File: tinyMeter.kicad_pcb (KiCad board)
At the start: 2 copper layers, 74.6 x 70 mm, 93 parts, among them J1 USB_MASTER, J2 DC_POWER, J3 USB_POWER, J4 USBA_OUT_2, J5 USBA_OUT_1, J6 DC_POWER, J7 Debug, J8 External antenna, Q1 100N03A, Q2 100N03A, Q3 100N03A, Q4 SS8050, SW1 SW_Push, SW2 SW_Push, SW3 SW_Push, SW4 SW_Push, SW5 SW_Push, SW6 Boot, SW7 Reset, U1 ESP32-S3, U2 INA219AxD, U3 INA219AxD, U4 INA219AxD, U5 AMS1117-3.3, Y1 Crystal_GND24

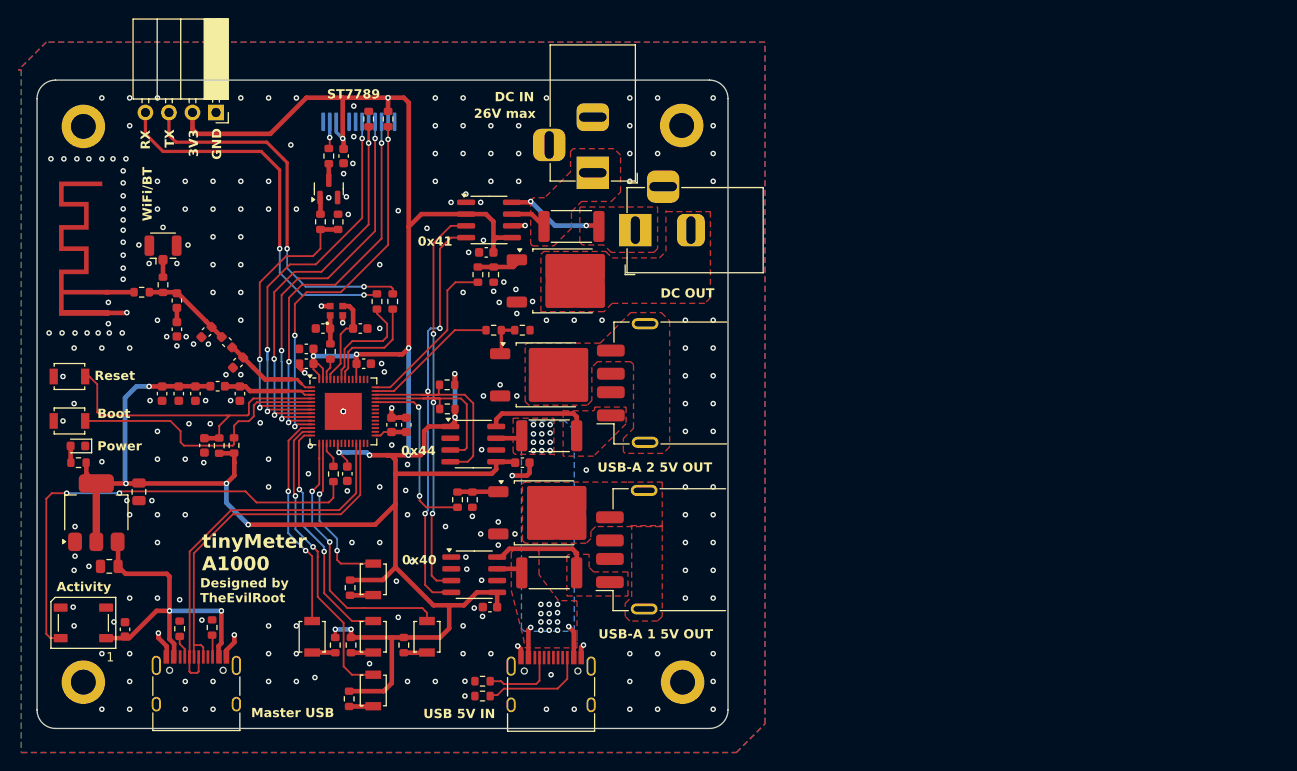
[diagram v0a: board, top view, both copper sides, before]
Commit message: Working on v2
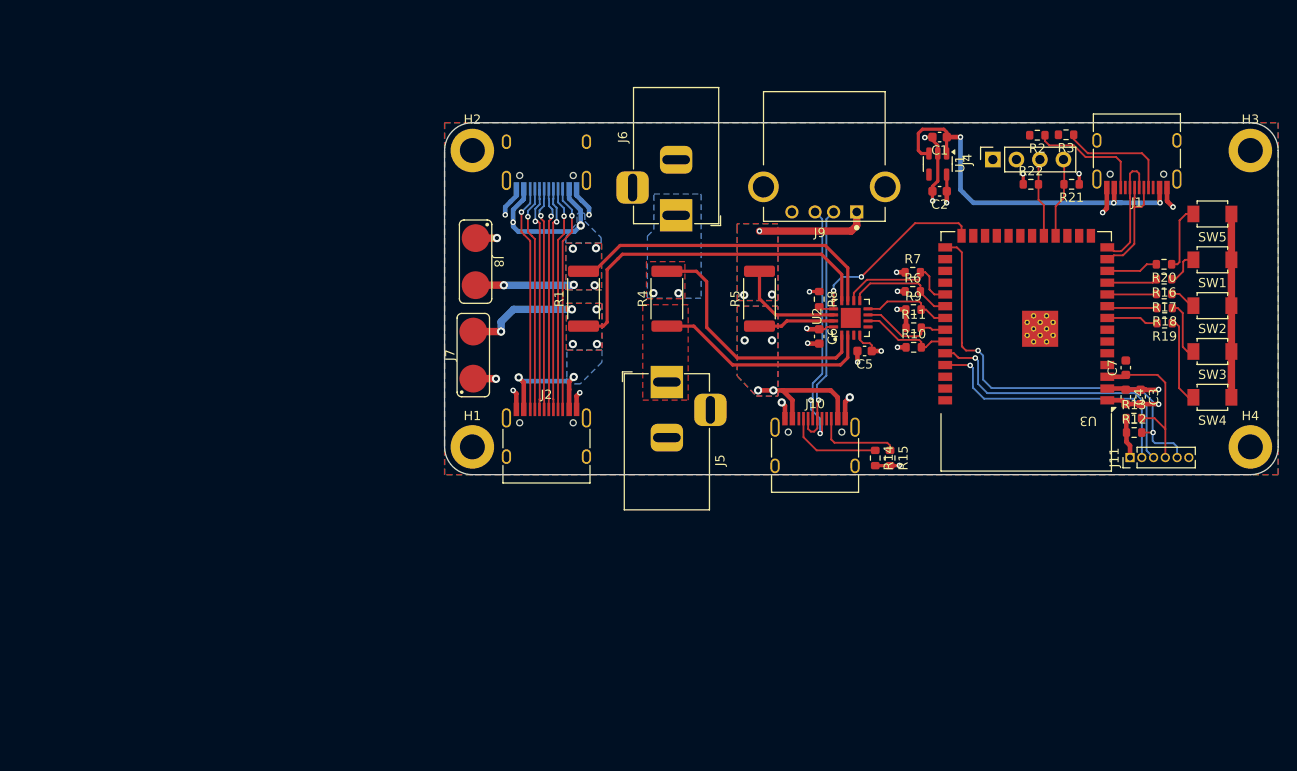
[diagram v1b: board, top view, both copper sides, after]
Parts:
- removed AE1: PCB antenna, Library:ESPRESSIF_ESP32_MIFA_2.4GHz_Right
- removed C10, C11, C16, C17, C19, C20, C21, C22, C23: 100n, Capacitor_SMD:C_0603_1608Metric
- removed C12, C15, C18: 1u, Capacitor_SMD:C_0603_1608Metric
- removed C13, C14: 10u, Capacitor_SMD:C_0603_1608Metric
- removed C8, C9: LNA, Capacitor_SMD:C_0603_1608Metric
- removed D1: WS2812B, LED_SMD:LED_WS2812B_PLCC4_5.0x5.0mm_P3.2mm
- removed D2: PWR_LED, LED_SMD:LED_0603_1608Metric
- removed DS1: ST77xx, Library:ST77XX
- removed L1, L2: L, Inductor_SMD:L_0603_1608Metric
- removed L3: 2n, Inductor_SMD:L_0603_1608Metric
- removed Q1, Q2, Q3: 100N03A, Package_TO_SOT_SMD:TO-252-2
- removed Q4: SS8050, Package_TO_SOT_SMD:SOT-23
- removed R23, R31: 1k, Resistor_SMD:R_0603_1608Metric
- removed R24, R25, R28, R32, R33, R34: 10k, Resistor_SMD:R_0603_1608Metric
- removed R26, R27: 2k7, Resistor_SMD:R_0603_1608Metric
- removed R29: 60, Resistor_SMD:R_0603_1608Metric
- removed R30: 100, Resistor_SMD:R_0603_1608Metric
- removed SW6: Boot, Button_Switch_SMD:SW_SPST_B3U-1000P
- removed SW7: Reset, Button_Switch_SMD:SW_SPST_B3U-1000P
- removed U4: INA219AxD, Package_SO:SOIC-8_3.9x4.9mm_P1.27mm
- removed U5: AMS1117-3.3, Package_TO_SOT_SMD:SOT-223-3_TabPin2
- removed Y1: Crystal_GND24, Library:OSC_XRCGB40M000F4M00R0
- added J10: USB_IN, TheEvilRoot:USB_C_Receptacle_HRO_TYPE-C-31-M-12, F.Cu at (223.0, 115.0)
- added J11: Conn_01x06, Connector_PinHeader_1.27mm:PinHeader_1x06_P1.27mm_Vertical, F.Cu at (257.0, 115.2)
- added J9: USB_OUT, TheEvilRoot:TE_292303-1, F.Cu at (227.5, 88.6)
- C1, C2: footprint Capacitor_SMD:C_0805_2012Metric -> Capacitor_SMD:C_0603_1608Metric
- C3: value 10u -> 1u
- C4, C5: value 10p -> 100n
- C6: value 10u -> 100n
- C7: value LNA -> 10u
- J1: value USB_MASTER -> USB_C_Receptacle_USB2.0_16P; footprint Connector_USB:USB_C_Receptacle_HRO_TYPE-C-31-M-12 -> TheEvilRoot:USB_C_Receptacle_HRO_TYPE-C-31-M-12
- J2: value DC_POWER -> USB_IN; footprint Connector_BarrelJack:BarrelJack_Horizontal -> TheEvilRoot:USB_C_Receptacle_HRO_TYPE-C-31-M-12
- J3: value USB_POWER -> USB_OUT; footprint Connector_USB:USB_C_Receptacle_HRO_TYPE-C-31-M-12 -> TheEvilRoot:USB_C_Receptacle_HRO_TYPE-C-31-M-12; moved to B.Cu
- J4: value USBA_OUT_2 -> OLED; footprint Connector_USB:USB_A_Receptacle_GCT_USB1046 -> Connector_PinSocket_2.54mm:PinSocket_1x04_P2.54mm_Vertical
- J5: value USBA_OUT_1 -> DC_IN; footprint Connector_USB:USB_A_Receptacle_GCT_USB1046 -> Connector_BarrelJack:BarrelJack_Horizontal
- J6: value DC_POWER -> DC_OUT
- J7: value Debug -> Conn_01x02; footprint Connector_PinSocket_2.54mm:PinSocket_1x04_P2.54mm_Horizontal -> TheEvilRoot:SolderWire-SMD-2pin-2.54mm-D3.0
- J8: value External antenna -> Conn_01x02; footprint Connector_Coaxial:U.FL_Hirose_U.FL-R-SMT-1_Vertical -> TheEvilRoot:SolderWire-SMD-2pin-2.54mm-D3.0
- R1, R4: value 5k1 -> R100; footprint Resistor_SMD:R_0603_1608Metric -> Resistor_SMD:R_2512_6332Metric
- R10, R6, R7, R9: value 0R -> 10k
- R11, R8: value R025 -> 10k; footprint Resistor_SMD:R_2512_6332Metric -> Resistor_SMD:R_0603_1608Metric
- R12, R13: value 220 -> 10k
- R14, R15: value 10k -> 5k1
- R16, R17, R18, R19: value 10k -> R
- R20: value 1k -> R
- R21: value 1k -> 2k7
- R22: value 10k -> 2k7
- R5: value R025 -> R100
- SW1: value SW_Push -> A1; footprint Button_Switch_SMD:SW_SPST_B3U-1000P -> TheEvilRoot:IT-1185AP
- SW2: value SW_Push -> A2; footprint Button_Switch_SMD:SW_SPST_B3U-1000P -> TheEvilRoot:IT-1185AP
- SW3: value SW_Push -> A3; footprint Button_Switch_SMD:SW_SPST_B3U-1000P -> TheEvilRoot:IT-1185AP
- SW4: value SW_Push -> A4; footprint Button_Switch_SMD:SW_SPST_B3U-1000P -> TheEvilRoot:IT-1185AP
- SW5: value SW_Push -> A0; footprint Button_Switch_SMD:SW_SPST_B3U-1000P -> TheEvilRoot:IT-1185AP
- U1: value ESP32-S3 -> AP2112K-3.3; footprint Package_DFN_QFN:QFN-56-1EP_7x7mm_P0.4mm_EP4x4mm -> Package_TO_SOT_SMD:SOT-23-5
- U2: value INA219AxD -> INA3221AIRGVR; footprint Package_SO:SOIC-8_3.9x4.9mm_P1.27mm -> TheEvilRoot:QFN65P400X400X100-17N
- U3: value INA219AxD -> ESP32-S3-WROOM-1; footprint Package_SO:SOIC-8_3.9x4.9mm_P1.27mm -> TheEvilRoot:ESP32-S3-WROOM-1
- moved H3 138.5 mm to (270.0, 82.0)
- moved J1 117.3 mm to (257.8, 82.0), turned to 180 degrees
- moved R13 114.1 mm to (257.4, 110.9), turned to 0 degrees
- moved R2 106.8 mm to (247.0, 80.3), turned to 180 degrees
- moved SW5 104.2 mm to (265.9, 88.8), turned to 180 degrees
- moved C3 101.2 mm to (258.1, 108.6)
- moved C1 100.9 mm to (236.4, 80.5)
- moved SW4 100.6 mm to (265.9, 108.7), turned to 180 degrees
- moved R18 97.6 mm to (260.8, 99.0), turned to 180 degrees
- moved R17 97.2 mm to (260.7, 97.5), turned to 180 degrees
- moved SW1 96.9 mm to (265.9, 93.8), turned to 180 degrees
- moved R16 96.3 mm to (260.7, 95.9), turned to 180 degrees
- moved C7 95.9 mm to (256.6, 105.5), turned to 90 degrees
- moved SW3 95.7 mm to (265.9, 103.7), turned to 180 degrees
- moved C2 92.3 mm to (236.4, 86.4), turned to 180 degrees
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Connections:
- C1 pad 1: USB_VBUS -> VBUS
- C3 pad 1: /ESP_EN -> +3V3
- C4 pad 1: /ESP_XTAL_N -> +3V3
- C5 pad 1: /ESP_XTAL_IN -> +3V3
- C7 pad 1: /ESP_LNA -> /ESP_EN
- J1 pad A4: USB_VBUS -> VBUS
- J1 pad A9: USB_VBUS -> VBUS
- J1 pad B4: USB_VBUS -> VBUS
- J1 pad B9: USB_VBUS -> VBUS
- J3 pad A4: PWR_5V -> /METER_1-
- J3 pad A5: /USB_POWER_CC1 -> /USB_C_CC1
- J3 pad A6: unconnected-(J3-D+-PadA6) -> /USB_C_D2+
- J3 pad A7: unconnected-(J3-D--PadA7) -> /USB_C_D1-
- J3 pad A8: unconnected-(J3-SBU1-PadA8) -> /USB_C_SBU1
- J3 pad A9: PWR_5V -> /METER_1-
- J3 pad B4: PWR_5V -> /METER_1-
- J3 pad B5: /USB_POWER_CC2 -> /USB_C_CC2
- J3 pad B6: unconnected-(J3-D+-PadB6) -> /USB_C_D1+
- J3 pad B7: unconnected-(J3-D--PadB7) -> /USB_C_D2-
- J3 pad B8: unconnected-(J3-SBU2-PadB8) -> /USB_C_SBU2
- J3 pad B9: PWR_5V -> /METER_1-
- J4 pad 1: /USBA_OUT2_VCC -> GND
- J4 pad 2: unconnected-(J4-D--Pad2) -> +3V3
- J4 pad 3: unconnected-(J4-D+-Pad3) -> /OLED_SCL
- J4 pad 4: /USBA_OUT2_GND -> /OLED_SDA
- J5 pad 1: /USBA_OUT1_VCC -> /METER_3+
- J5 pad 2: unconnected-(J5-D--Pad2) -> GND
- J5 pad 3: unconnected-(J5-D+-Pad3) -> (no net)
- J6 pad 1: /DC_POWER_VCC -> /METER_3-
- J6 pad 2: /DC_POWER_GND -> GND
- J7 pad 2: +3V3 -> /METER_1+
- J8 pad 1: /WIFI_ANTENNA_EXT -> GND
- J8 pad 2: GND -> /METER_1-
- R1 pad 1: GND -> /METER_1+
- R1 pad 2: /USB_MASTER_CC2 -> /METER_1-
- R10 pad 1: /WIFI_ANTENNA -> +3V3
- R10 pad 2: /WIFI_ANTENNA_EXT -> /METER_SCL
- R11 pad 1: /DC_POWER_VCC -> +3V3
- R11 pad 2: PWR_DC -> /METER_SDA
- R12 pad 1: /MCU_LED_DIN -> +3V3
- R12 pad 2: /MCU_LED_DATA -> /ESP_BOOT
- R13 pad 2: /3V3_PWR_LED -> /ESP_EN
- R14 pad 1: Net-(R14-Pad1) -> /USB_A_CC1
- R14 pad 2: +3V3 -> GND
- R15 pad 1: Net-(R15-Pad1) -> /USB_A_CC2
- R15 pad 2: +3V3 -> GND
- R16 pad 2: +3V3 -> /SW_A1
- R17 pad 2: +3V3 -> /SW_A2
- R18 pad 2: +3V3 -> /SW_A3
- R19 pad 1: /USBA_OUT1_GATE -> Net-(R19-Pad1)
- R19 pad 2: GND -> /SW_A4
- R2 pad 1: GND -> /USB_MASTER_CC2
- R2 pad 2: /USB_MASTER_CC1 -> GND
- R20 pad 1: /USBA_OUT1_GATE -> Net-(R20-Pad1)
- R20 pad 2: /USBA_OUT_1_FETGATE -> /SW_A0
- R21 pad 1: /USBA_OUT2_GATE -> +3V3
- R21 pad 2: /USBA_OUT_2_FETGATE -> /OLED_SDA
- R22 pad 1: /USBA_OUT2_GATE -> +3V3
- R22 pad 2: GND -> /OLED_SCL
- R3 pad 1: GND -> /USB_MASTER_CC1
- R3 pad 2: /USB_POWER_CC2 -> GND
- R4 pad 1: GND -> /METER_3+
- R4 pad 2: /USB_POWER_CC1 -> /METER_3-
- R5 pad 1: /USBA_OUT1_VCC -> /METER_2+
- R5 pad 2: PWR_5V -> /METER_2-
- R6 pad 1: /ESP_TX -> +3V3
- R6 pad 2: /ESP_TDX0 -> /METER_CRIT
- R7 pad 1: /ESP_RX -> +3V3
- R7 pad 2: /ESP_RDX0 -> /METER_VALID
- R8 pad 1: /USBA_OUT2_VCC -> +3V3
- R8 pad 2: PWR_5V -> /METER_TIMING
- R9 pad 1: /WIFI_ANTENNA -> +3V3
- R9 pad 2: /WIFI_ANTENNA_PCB -> /METER_WARN
- SW1 pad 1: /KEYPAD_K1 -> +3V3
- SW1 pad 2: Net-(R14-Pad1) -> Net-(R16-Pad1)
- SW2 pad 1: /KEYPAD_K2 -> +3V3
- SW2 pad 2: Net-(R15-Pad1) -> Net-(R17-Pad1)
- SW3 pad 1: /KEYPAD_K3 -> +3V3
- SW3 pad 2: Net-(R16-Pad1) -> Net-(R18-Pad1)
- SW4 pad 1: /KEYPAD_K4 -> +3V3
- SW4 pad 2: Net-(R17-Pad1) -> Net-(R19-Pad1)
- SW5 pad 1: /KEYPAD_K5 -> +3V3
- SW5 pad 2: Net-(R18-Pad1) -> Net-(R20-Pad1)
- U1 pad 1: /ESP_LNA -> VBUS
- U1 pad 2: /ESP_VDD_3P3 -> GND
- U1 pad 3: /ESP_VDD_3P3 -> VBUS
- U1 pad 4: /ESP_EN -> unconnected-(U1-NC-Pad4)
- U1 pad 5: /ESP_IO0 -> +3V3
- U2 pad 1: GND -> /METER_3-
- U2 pad 2: GND -> /METER_3+
- U2 pad 3: /METER_SDA -> GND
- U2 pad 4: /METER_SCL -> +3V3
- U2 pad 5: +3V3 -> GND
- U2 pad 6: GND -> /METER_SCL
- U2 pad 7: PWR_5V -> /METER_SDA
- U2 pad 8: /USBA_OUT1_VCC -> /METER_WARN
- U3 pad 1: +3V3 -> GND
- U3 pad 2: GND -> +3V3
- U3 pad 3: /METER_SDA -> /ESP_EN
- U3 pad 4: /METER_SCL -> unconnected-(U3-IO4-Pad4)
- U3 pad 5: +3V3 -> unconnected-(U3-IO5-Pad5)
- U3 pad 6: GND -> unconnected-(U3-IO6-Pad6)
- U3 pad 7: PWR_5V -> unconnected-(U3-IO7-Pad7)
- U3 pad 8: /USBA_OUT2_VCC -> /SW_A4
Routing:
- net +3V3: track 280.1 -> 48.9 mm, vias 16 -> 11
- net /METER_1+: track 0.00 -> 64.1 mm, vias 0 -> 7
- net /METER_1-: track 0.00 -> 60.5 mm, vias 0 -> 7
- net /METER_SCL: track 66.8 -> 10.1 mm, vias 3 -> 0
- net /METER_SDA: track 62.7 -> 10.2 mm, vias 3 -> 0
- net /MCU_LED_DIN: track 50.1 -> 0.00 mm, vias 2 -> 0
- net /ESP_BOOT: track 0.00 -> 46.5 mm, vias 0 -> 2
- net /DISPLAY_CS: track 43.4 -> 0.00 mm, vias 3 -> 0
- net /DISPLAY_DC: track 43.1 -> 0.00 mm, vias 3 -> 0
- net /DISPLAY_RST: track 42.6 -> 0.00 mm, vias 3 -> 0
- net VBUS: track 0.00 -> 42.3 mm, vias 0 -> 3
- net /DISPLAY_SCK: track 41.4 -> 0.00 mm, vias 3 -> 0
- net /DISPLAY_SDA: track 41.3 -> 0.00 mm, vias 3 -> 0
- net USB_VBUS: track 37.1 -> 0.00 mm, vias 2 -> 0
- net /KEYPAD_K5: track 32.5 -> 0.00 mm, vias 2 -> 0
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- added copper zone on In2.Cu, net +3V3
- added copper zone on B.Cu, net /METER_1+
- added copper zone on F.Cu, net /METER_1+
- added copper zone on B.Cu, net /METER_1-
- added copper zone on F.Cu, net /METER_1-
- added copper zone on B.Cu, net /METER_2+
- added copper zone on F.Cu, net /METER_2+
- added copper zone on B.Cu, net /METER_2-
- added copper zone on F.Cu, net /METER_2-
- added copper zone on F.Cu, net /METER_3+
- added copper zone on B.Cu, net /METER_3-
- added copper zone on F.Cu, net /METER_3-
- added copper zone on In1.Cu, net GND
- removed copper zone on F.Cu, net /DC_POWER_GND
- removed copper zone on F.Cu, net /DC_POWER_VCC
- removed copper zone on F.Cu, net /USBA_OUT1_GND
- removed copper zone on F.Cu, net /USBA_OUT1_VCC
- removed copper zone on F.Cu, net /USBA_OUT2_GND
- removed copper zone on F.Cu, net /USBA_OUT2_VCC
- removed copper zone on B.Cu, net PWR_5V
- removed copper zone on F.Cu, net PWR_5V
- removed copper zone on F.Cu, net PWR_DC
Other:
- board size 74.6 x 70 mm -> 90 x 38 mm
- copper layers 2 -> 4
- board text removed: "0x40"
- board text removed: "0x41"
- board text removed: "0x44"
- board text removed: "26V max"
- board text removed: "3V3"
- board text removed: "Activity"
- board text removed: "Boot"
- board text removed: "DC IN"
- board text removed: "DC OUT"
- board text removed: "Designed by TheEvilRoot"
- board text removed: "GND"
- board text removed: "Master USB"
- board text removed: "Power"
- board text removed: "RX"
- board text removed: "Reset"
- board text removed: "ST7789"
- board text removed: "TX"
- board text removed: "USB 5V IN"
- board text removed: "USB-A 1 5V OUT"
- board text removed: "USB-A 2 5V OUT"
- board text removed: "WiFi/BT"
- board text removed: "tinyMeter A1000"
